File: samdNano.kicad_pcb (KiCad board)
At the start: 2 copper layers, 50.8 x 17.8 mm, 34 parts, among them J1 Analog, J2 Digital, J3 USB-C, J4 J Link, SW1 RESET, U1 AMS1117-3.3, U2 ATSAMD21G18A-A, Y1 32.768 kHz

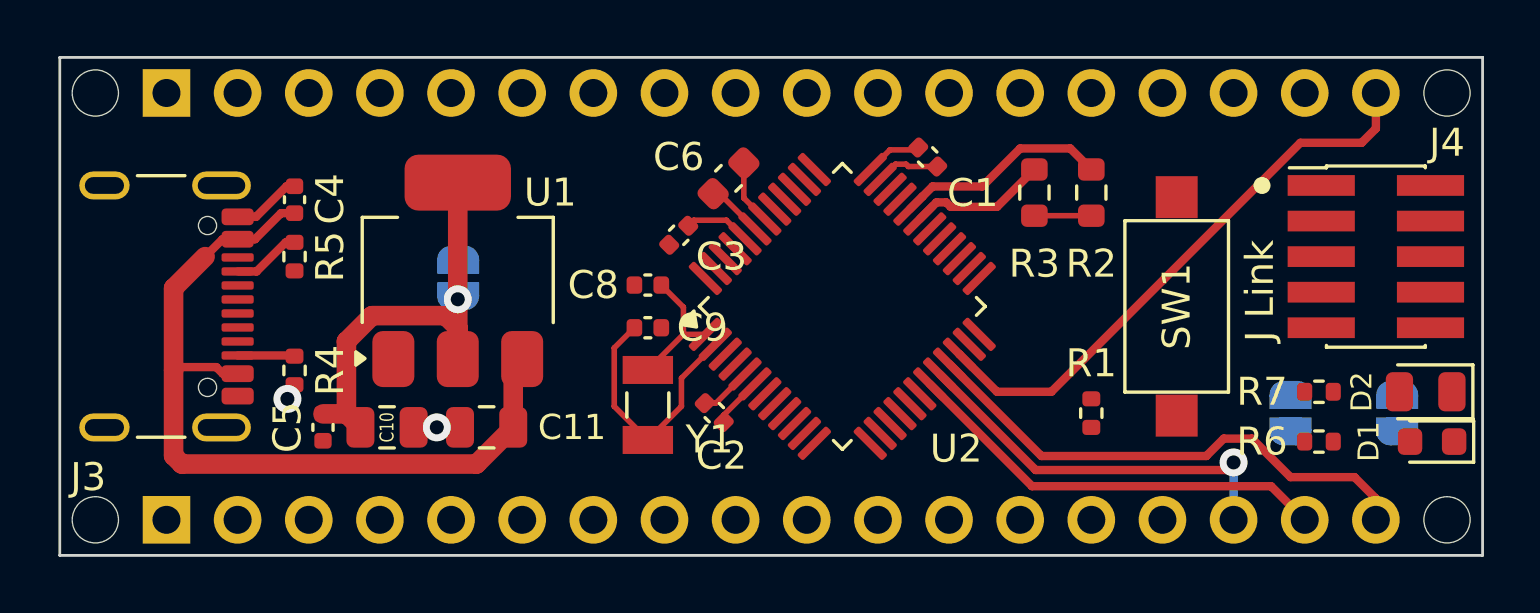
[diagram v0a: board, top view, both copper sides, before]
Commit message: commit
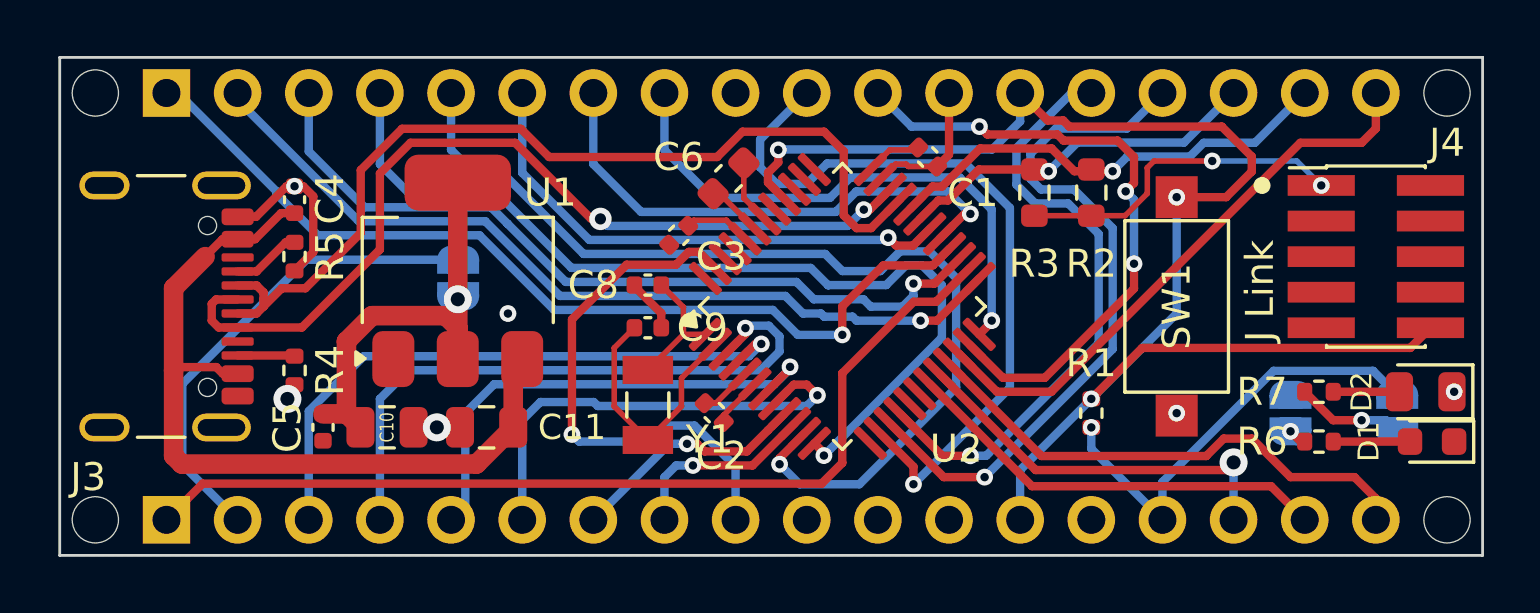
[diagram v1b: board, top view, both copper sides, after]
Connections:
- J1 pad 15: +3V3 -> +3.3V
- J1 pad 2: +3V3 -> +3.3V
- J2 pad 14: DO -> D0
- U2 pad 10: unconnected-(U2-PA05-Pad10) -> A4
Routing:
- net RST: track 0.00 -> 52.0 mm, vias 0 -> 3
- net +3.3V: track 8.28 -> 51.6 mm, vias 0 -> 3
- net D8: track 0.00 -> 36.0 mm, vias 0 -> 1
- net D13: track 0.00 -> 34.3 mm
- net D12: track 0.00 -> 33.5 mm, vias 0 -> 1
- net D9: track 0.00 -> 33.4 mm, vias 0 -> 1
- net D-: track 0.00 -> 33.2 mm
- net D+: track 0.00 -> 32.0 mm, vias 0 -> 2
- net D11: track 0.00 -> 30.6 mm, vias 0 -> 1
- net D10: track 0.00 -> 28.7 mm, vias 0 -> 1
- net D3: track 0.00 -> 27.1 mm, vias 0 -> 1
- net D1: track 0.00 -> 25.1 mm, vias 0 -> 1
- net D2: track 0.00 -> 22.7 mm, vias 0 -> 3
- net A0: track 0.00 -> 22.5 mm, vias 0 -> 1
- net AREF: track 0.00 -> 22.3 mm, vias 0 -> 1
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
